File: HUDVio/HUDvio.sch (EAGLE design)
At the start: 70 parts, among them J2 PHOENIX_SPTAF1/2-3,5, U1 ST_STM32F446RET7, U3 TVP5150AM1PBSR, U4 NEXPERIA_NVT2006, U5 MAXIM_MAX4389, U6 MIC_MIC5504-1.8, U7 TOR_XC6220B331, U8 ROHM_BD50HC5WEFJ, X1 ABRACON_ABM8-27.000MHZ, X2 ABRACON_ABM8-14.31818MHZ

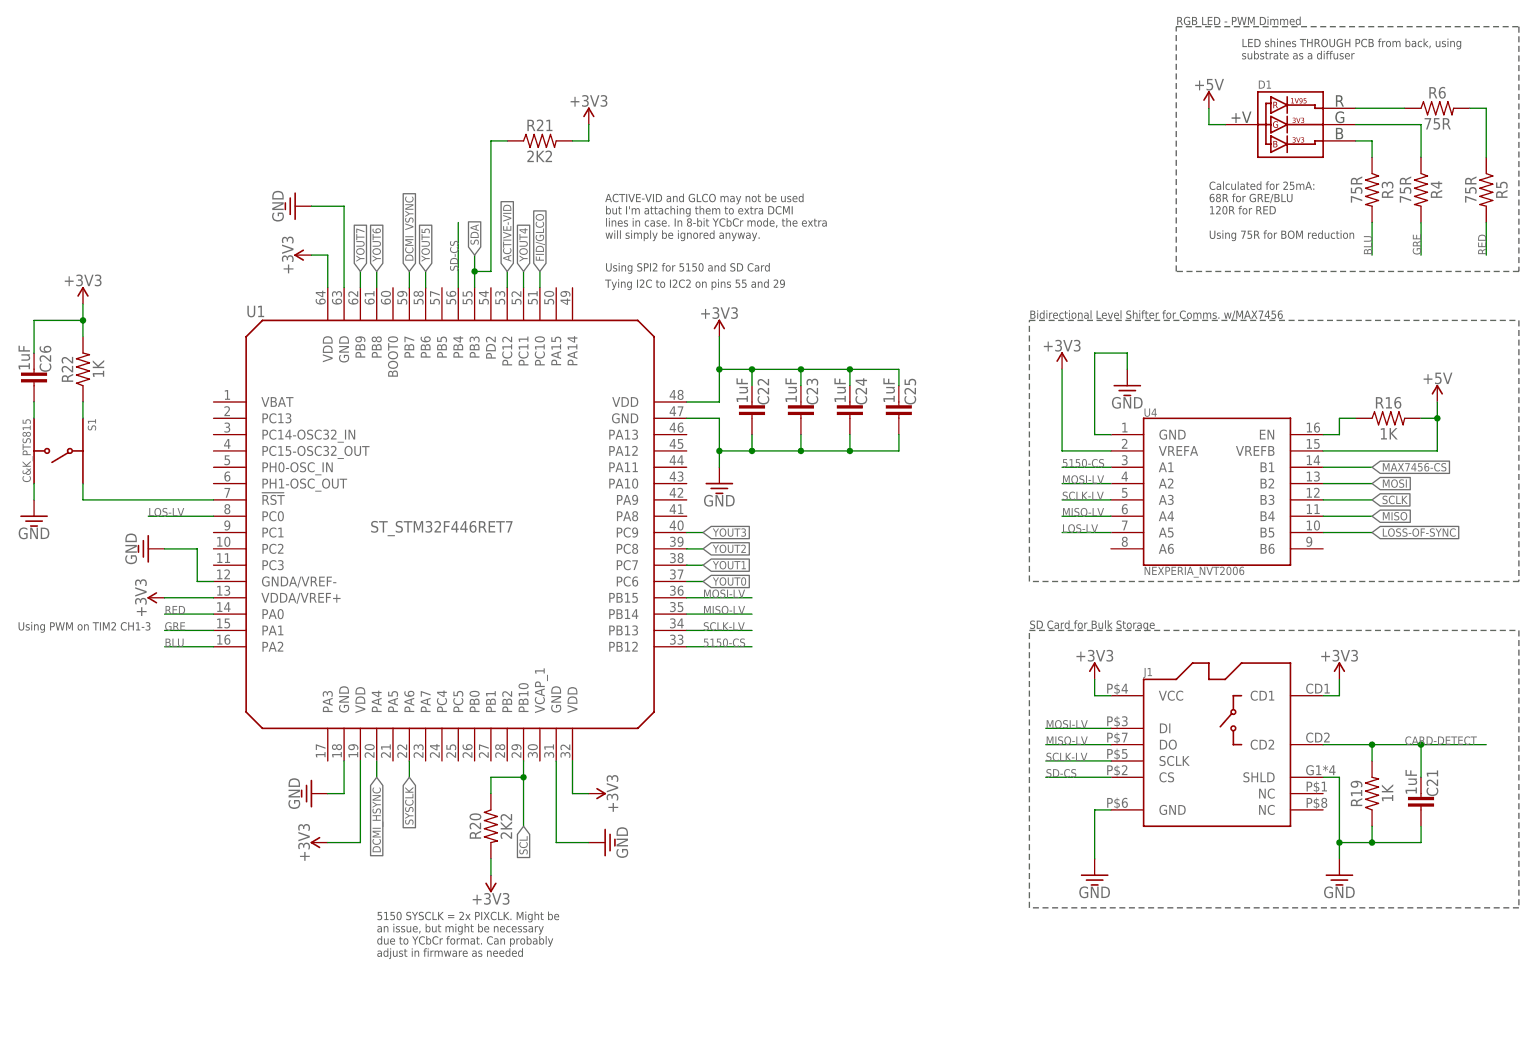
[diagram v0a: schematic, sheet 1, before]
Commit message: Schematic Complete
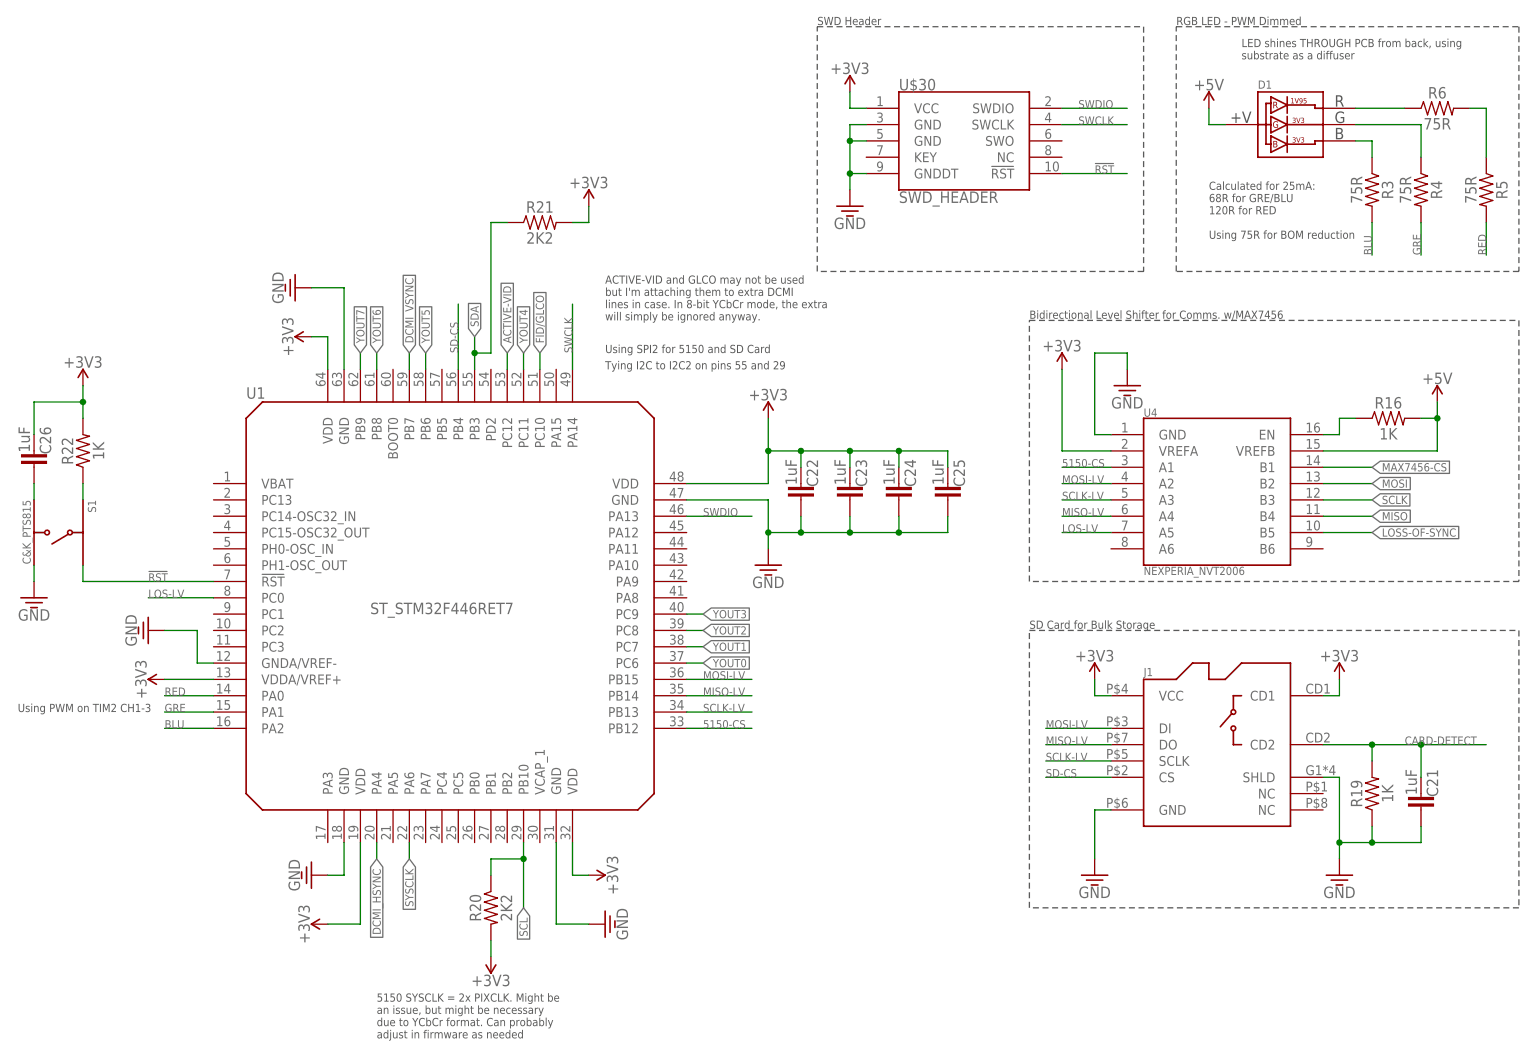
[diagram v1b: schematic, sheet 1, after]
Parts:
- added U$30: SWD_HEADER, Skyhawkson-Connectors:SWD_HEADER
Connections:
- removed net N$16: S1.2, U1.!RST!@7
- new net !RST: S1.2, U$30.!RST!@10, U1.!RST!@7
- new net SWCLK: U$30.SWCLK@4, U1.PA14@49
- new net SWDIO: U$30.SWDIO@2, U1.PA13@46
- net +3V3: now also U$30.VCC@1
- net GND: now also U$30.GND@3, U$30.GND@5, U$30.GNDDT@9
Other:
- note added: "SWD Header"
- moved on the sheet: C22, C23, C24, C25, C26, R20, R21, R22, S1, U1
